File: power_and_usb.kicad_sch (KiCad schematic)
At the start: 9 parts, among them J1 USB4085-GF-A_REVB, U1 USBLC6-2SC6, U2 MCP1755T-3302E/DC

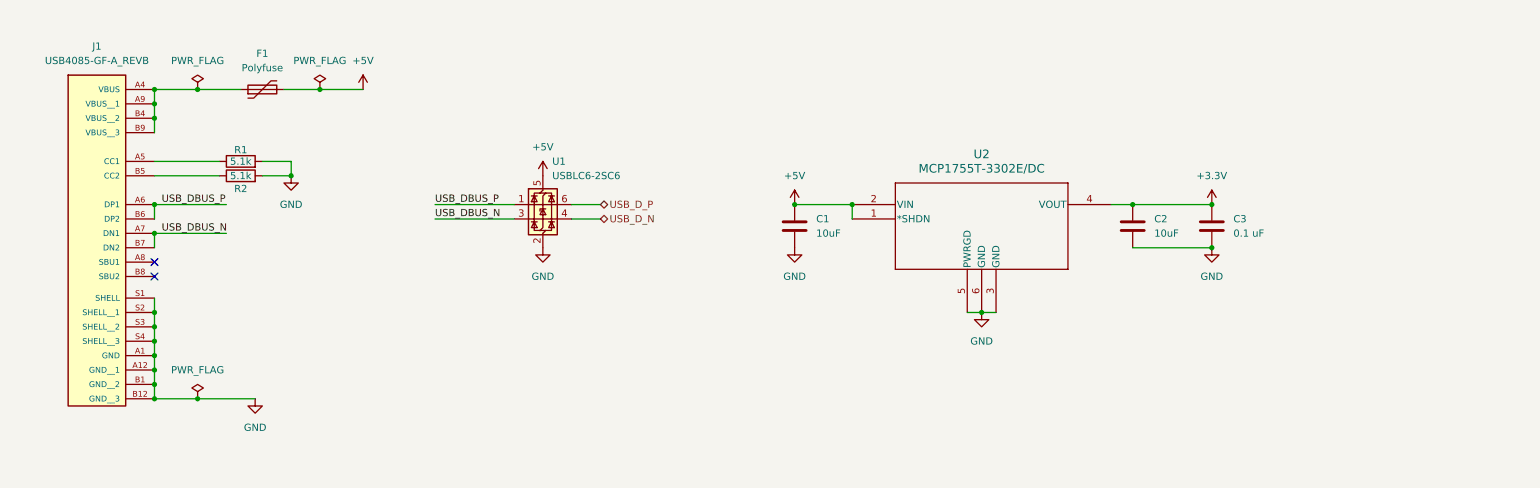
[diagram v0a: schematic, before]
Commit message: power documentation
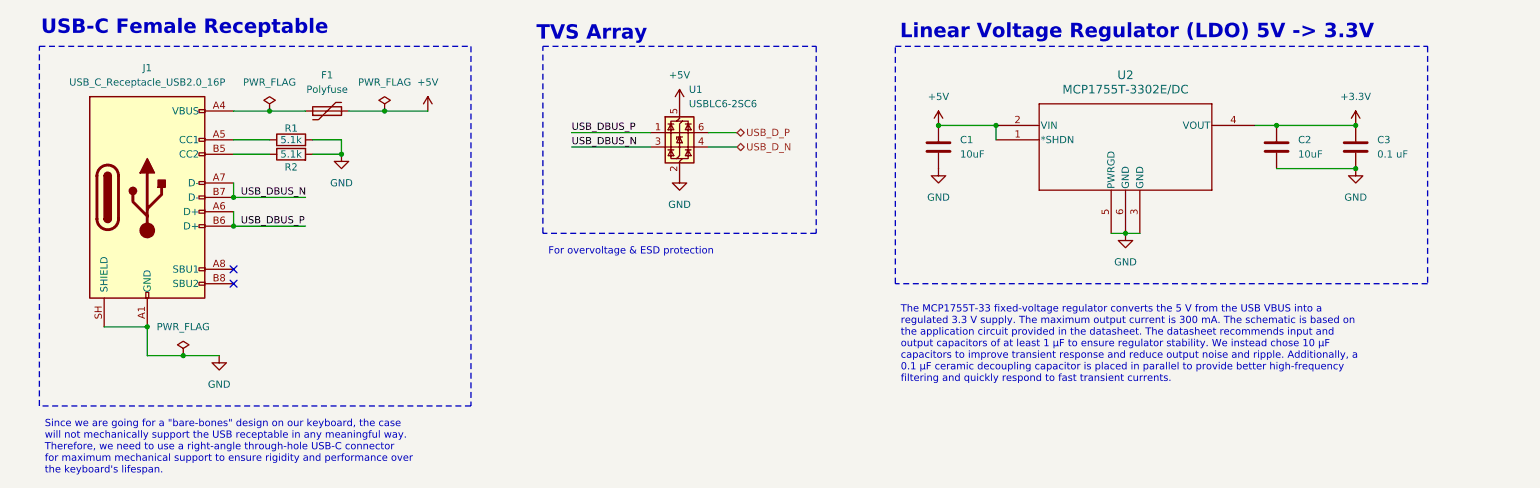
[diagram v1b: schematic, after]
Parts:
- removed J1: USB4085-GF-A_REVB, USB4085-GF-A_REVB:GCT_USB4085-GF-A_REVB, symbol KeyboardSymbols:USB4085-GF-A_REVB
- added J1: USB_C_Receptacle_USB2.0_16P, symbol Connector:USB_C_Receptacle_USB2.0_16P
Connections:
- net GND: now also J1.A1 (GND), J1.A12 (GND), J1.B1 (GND), J1.B12 (GND), J1.SH (SHIELD)
- net USB_DBUS_N: now also J1.A7 (D-), J1.B7 (D-)
- net USB_DBUS_P: now also J1.A6 (D+), J1.B6 (D+)
- net at F1.1: now also J1.A4 (VBUS), J1.A9 (VBUS), J1.B4 (VBUS), J1.B9 (VBUS)
- net at R1.1: now also J1.A5 (CC1)
- net at R2.1: now also J1.B5 (CC2)
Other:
- note added: "Linear Voltage Regulator (LDO) 5V -> 3.3V"
- note added: "TVS Array"
- note added: "USB-C Female Receptable"
- moved on the sheet: C1, C2, C3, F1, R1, R2, U1, U2
